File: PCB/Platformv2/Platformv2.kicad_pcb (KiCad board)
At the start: 2 copper layers, 122.5 x 92 mm, 36 parts, among them J1 Program, J10 Pin_SERIAL, J12 Pin_DIO_LORA, J2 Conn_01x02_Pin, J3 Conn_01x02_Pin, J4 Pin_SIM800L, J5 Pin_RTC, J6 Micro_SD_Card, J7 Pin_Analog, J8 Pin_SPI_1, J9 Pin_I2C_eksternal, SW1 SW_Push, SW2 SW_Push, SW3 RST, U1 SIM800L-CORE, U2 MAX485_MODULE_5V_LOGIC_TLL_TO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, U3 Ai-Thinker-Ra-02, U4 AMS1117CD-3.3

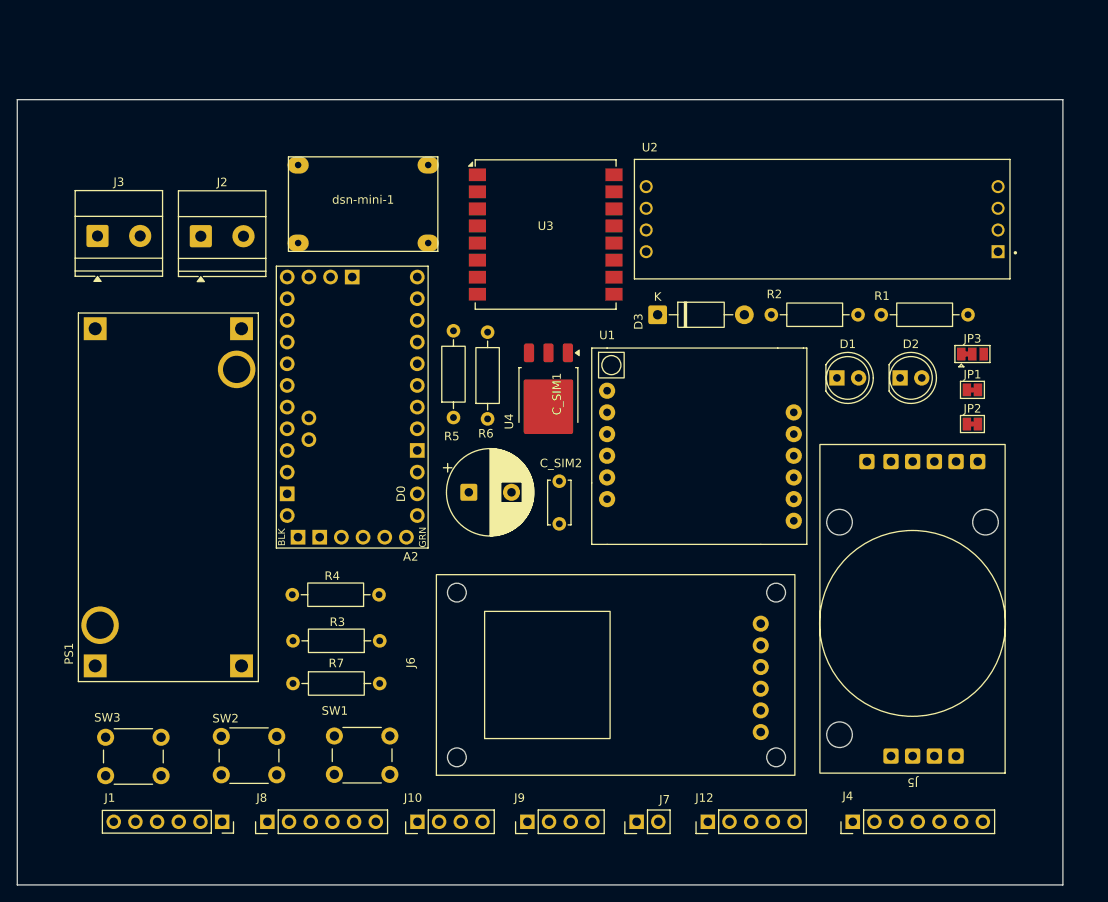
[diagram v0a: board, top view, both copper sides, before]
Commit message: Update 8 Oktober 2026
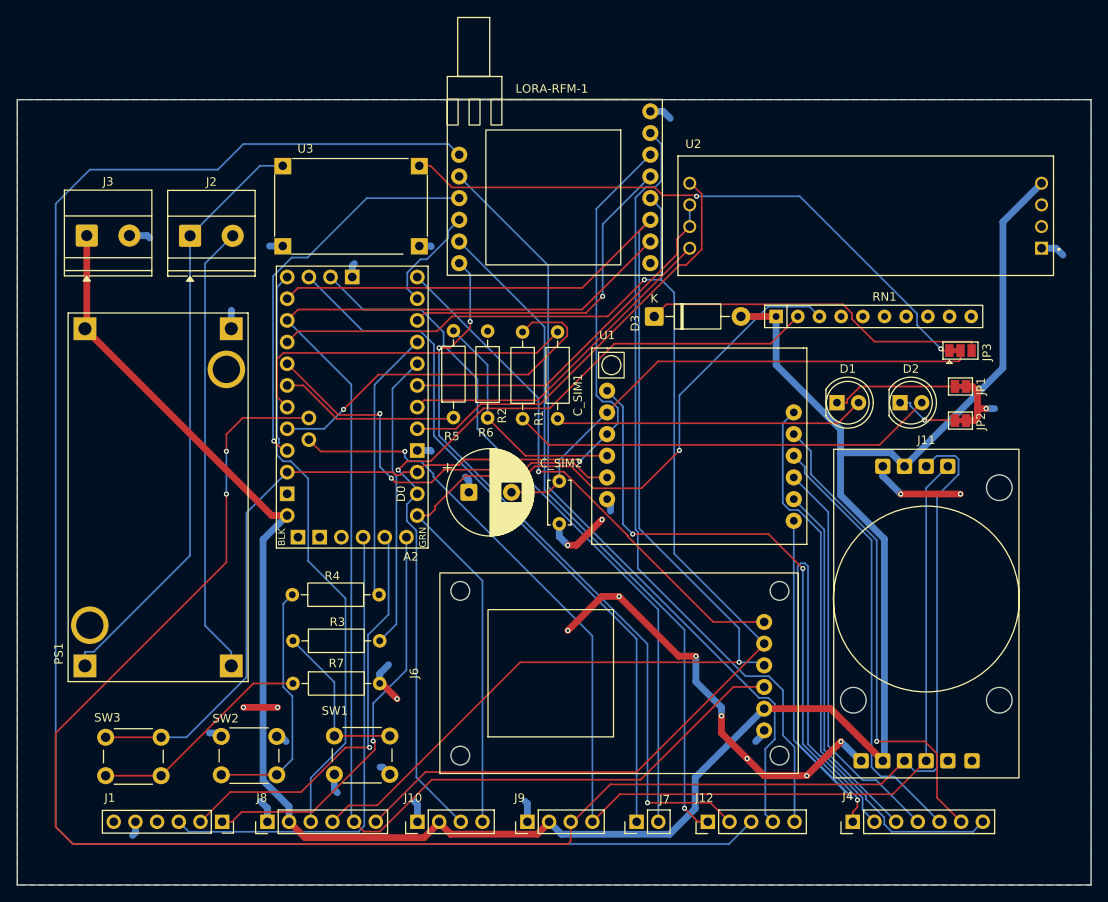
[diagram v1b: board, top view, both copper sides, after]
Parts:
- removed J5: Pin_RTC, DS3231:DS3231
- removed U4: AMS1117CD-3.3, Package_TO_SOT_SMD:TO-252-3_TabPin2
- removed dsn-mini-1: ~, Mini360_step-down:Mini360_step-down
- added J11: Pin_RTC, DS3231:DS3231, F.Cu at (162.0, 93.0)
- added LORA-RFM-1: ~, lora_module:lora, F.Cu at (105.9, 32.8)
- added RN1: R_Network09_US, Resistor_THT:R_Array_SIP10, F.Cu at (144.4, 58.2)
- U3: value Ai-Thinker-Ra-02 -> ~; footprint RF_Module:Ai-Thinker-Ra-01-LoRa -> Mini360_step_down_converter:Untitled
- moved R1 48.1 mm to (118.8, 60.0), turned to -90 degrees
- moved R2 39.4 mm to (114.7, 60.0), turned to -90 degrees
- moved U3 23.1 mm to (94.5, 45.3)
- moved U2 5.12 mm to (154.9, 46.4)
- moved D1 2.90 mm to (151.5, 68.3)
- moved D2 2.90 mm to (158.9, 68.3)
- moved JP3 1.46 mm to (166.0, 62.2)
- moved JP1 1.46 mm to (166.0, 66.4)
- moved JP2 1.46 mm to (166.0, 70.4)
- moved J3 1.26 mm to (63.6, 48.7)
- moved J2 1.26 mm to (75.7, 48.8)
- moved PS1 1.20 mm to (72.0, 79.4)
- moved D3 0.45 mm to (130.1, 58.2)
- moved J6 0.45 mm to (126.0, 100.0)
- moved R6 0.12 mm to (110.6, 70.1)
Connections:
- A2 pad RAW: unconnected-(A2-PadRAW) -> +5V
- A2 pad Vcc1: +5V -> +3.3V
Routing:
- net +5V: track 0.00 -> 275.3 mm
- net /I2C_UART_BUS.SDA: track 0.00 -> 216.5 mm, vias 0 -> 2
- net /LORA_DIO3: track 0.00 -> 207.1 mm
- net /SPI_BUS.MISO: track 0.00 -> 163.9 mm
- net /SPI_BUS.MOSI: track 0.00 -> 162.1 mm, vias 0 -> 1
- net /SPI_BUS.SCK: track 0.00 -> 158.8 mm, vias 0 -> 1
- net /I2C_UART_BUS.SCL: track 0.00 -> 142.7 mm, vias 0 -> 1
- net GND: track 0.00 -> 125.3 mm, vias 0 -> 15
- net /RST: track 0.00 -> 122.8 mm, vias 0 -> 1
- net /I2C_UART_BUS.RX: track 0.00 -> 102.9 mm, vias 0 -> 1
- net /SIM_SPK-: track 0.00 -> 99.9 mm
- net /I2C_UART_BUS.TX: track 0.00 -> 99.5 mm, vias 0 -> 1
- net /LORA_DIO5: track 0.00 -> 92.4 mm
- net /LORA_DIO4: track 0.00 -> 92.4 mm
- net /LORA_DIO2: track 0.00 -> 86.7 mm, vias 0 -> 3
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- added copper zone on B.Cu, net GND
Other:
- board size 122.5 x 92 mm -> 125.8 x 92 mm
